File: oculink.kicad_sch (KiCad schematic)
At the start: 10 parts, among them J3 OCuLink_x4_Amphenol_G14A42121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, J4 OCuLink_x4_Amphenol_G14A42121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, J5 OCuLink_x4_Amphenol_G14A42121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

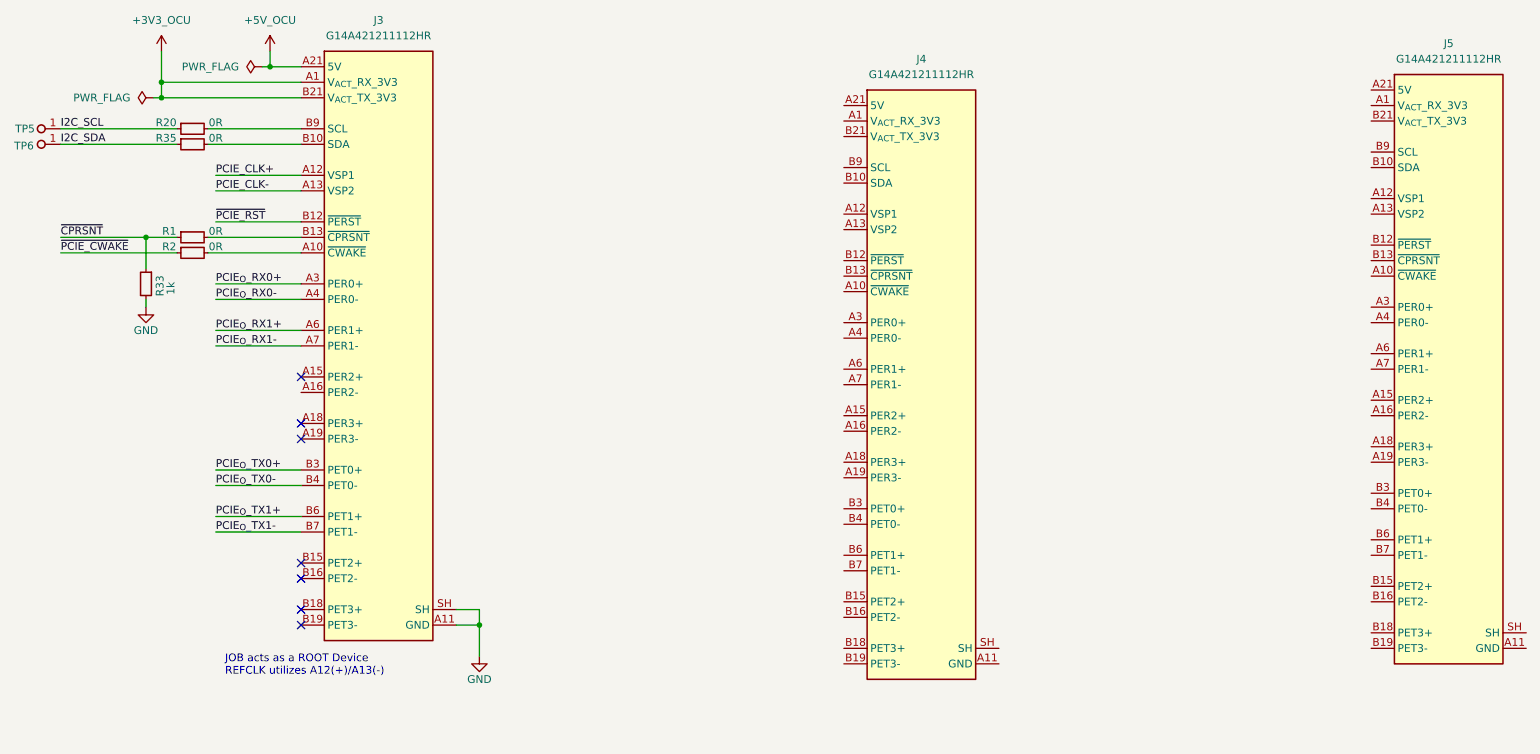
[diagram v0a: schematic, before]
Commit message: [#100765] Update subsheets
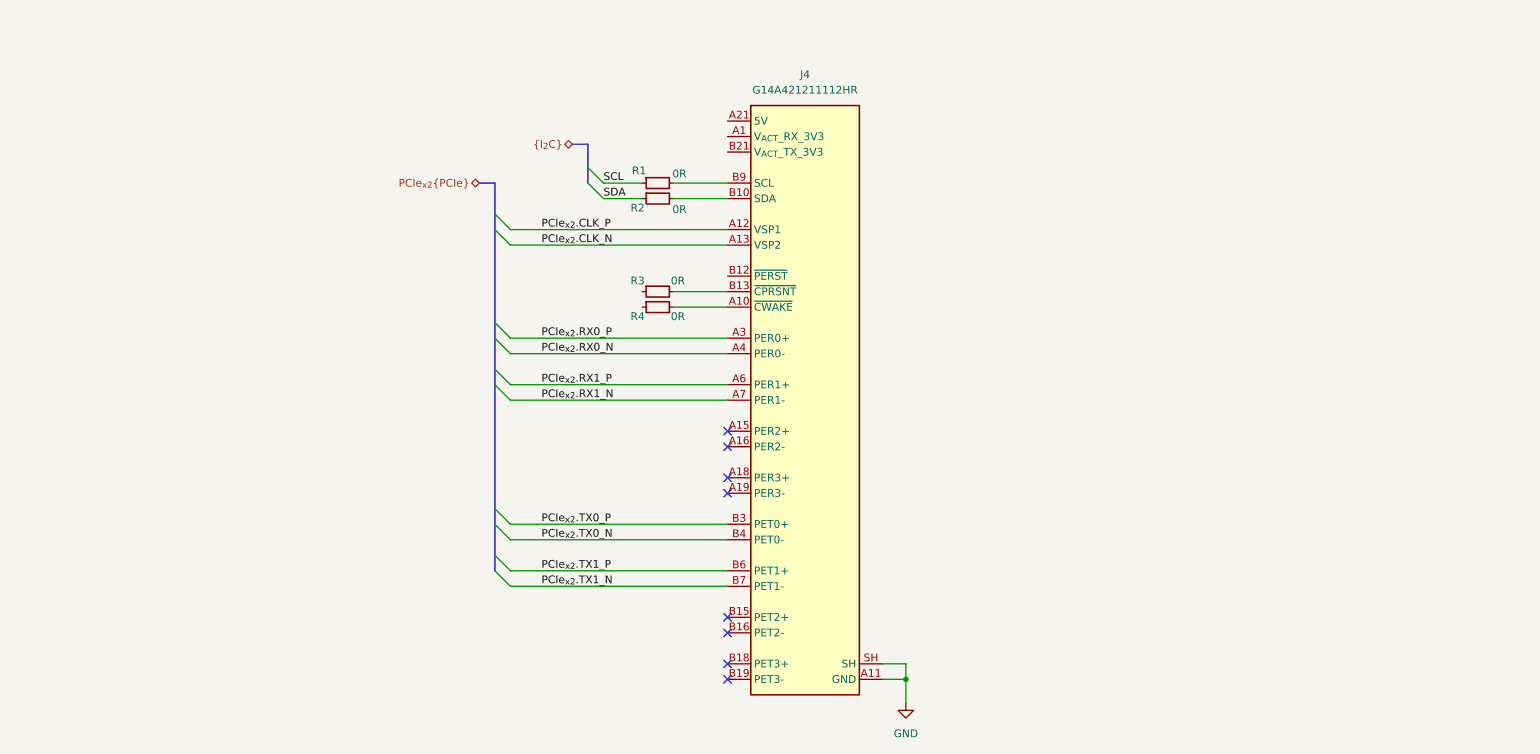
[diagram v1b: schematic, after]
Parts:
- removed J3, J5: OCuLink_x4_Amphenol_G14A421211112HR, antmicro-footprints:Amphenol_G14A421211112HR, symbol antmicroPciConnectors:OCuLink_x4_Amphenol_G14A421211112HR
- removed R20, R35: R_0R_0402, antmicro-footprints:R_0402_1005Metric, symbol antmicroResistors0402:R_0R_0402
- removed R33: R_1k_0402, antmicro-footprints:R_0402_1005Metric, symbol antmicroResistors0402:R_1k_0402
- removed TP5, TP6: TP_1.5mm_SMD, antmicro-footprints:TP_SMD_1.5mm, symbol antmicroTestPoints:TP_1.5mm_SMD
- added R3, R4: R_0R_0402, antmicro-footprints:R_0402_1005Metric, symbol antmicroResistors0402:R_0R_0402
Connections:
- net GND: now also J4.A11 (GND), J4.A14 (GND), J4.A17 (GND), J4.A2 (GND), J4.A20 (GND), J4.A5 (GND), J4.A8 (GND), J4.B11 (GND), J4.B14 (GND), J4.B17 (GND), J4.B2 (GND), J4.B20 (GND), J4.B5 (GND), J4.B8 (GND), J4.SH
- net at R2.2: now also J4.B10 (SDA)
- net at R1.2: now also J4.B9 (SCL)
- net at J4.A10 (~{CWAKE}): now also R4.2
- net PCIe_{x2}.CLK_P: now reaches J4.A12 (VSP1)
- net PCIe_{x2}.CLK_N: now reaches J4.A13 (VSP2)
- net PCIe_{x2}.RX0_P: now reaches J4.A3 (PER0+)
- net PCIe_{x2}.RX0_N: now reaches J4.A4 (PER0-)
- net PCIe_{x2}.RX1_P: now reaches J4.A6 (PER1+)
- net PCIe_{x2}.RX1_N: now reaches J4.A7 (PER1-)
- net at J4.B13 (~{CPRSNT}): now also R3.2
- net PCIe_{x2}.TX0_P: now reaches J4.B3 (PET0+)
- net PCIe_{x2}.TX0_N: now reaches J4.B4 (PET0-)
- net PCIe_{x2}.TX1_P: now reaches J4.B6 (PET1+)
- net PCIe_{x2}.TX1_N: now reaches J4.B7 (PET1-)
- net ~{CPRSNT} renamed SCL
- net ~{PCIE_CWAKE} renamed SDA
- no-connect marks 7 -> 8
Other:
- note removed: "JOB acts as a ROOT Device REFCLK utilizes A12(+)/A13(-)"
- moved on the sheet: J4
